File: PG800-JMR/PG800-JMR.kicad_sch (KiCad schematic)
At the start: 51 parts, among them J1 DIN-6, J10 POT_POWER_2, J11 POT_POWER_3, J2 POT_CENTERS_1, J3 POT_CENTERS_2, J4 POT_CENTERS_3, J5 SWITCH_BLK, J6 TEENSY_PIN_BLK1, J7 TEENSY_PIN_BLK3, J8 TEENSY_PIN_BLK2, J9 POT_POWER_1, Q1 BSS138, Q2 BSS138, Q3 BSS138, U1 LM2575-5BT, U2 CD74HC4067M, U3 CD74HC4067M, U4 CD74HC4067M, U5 74HC165A

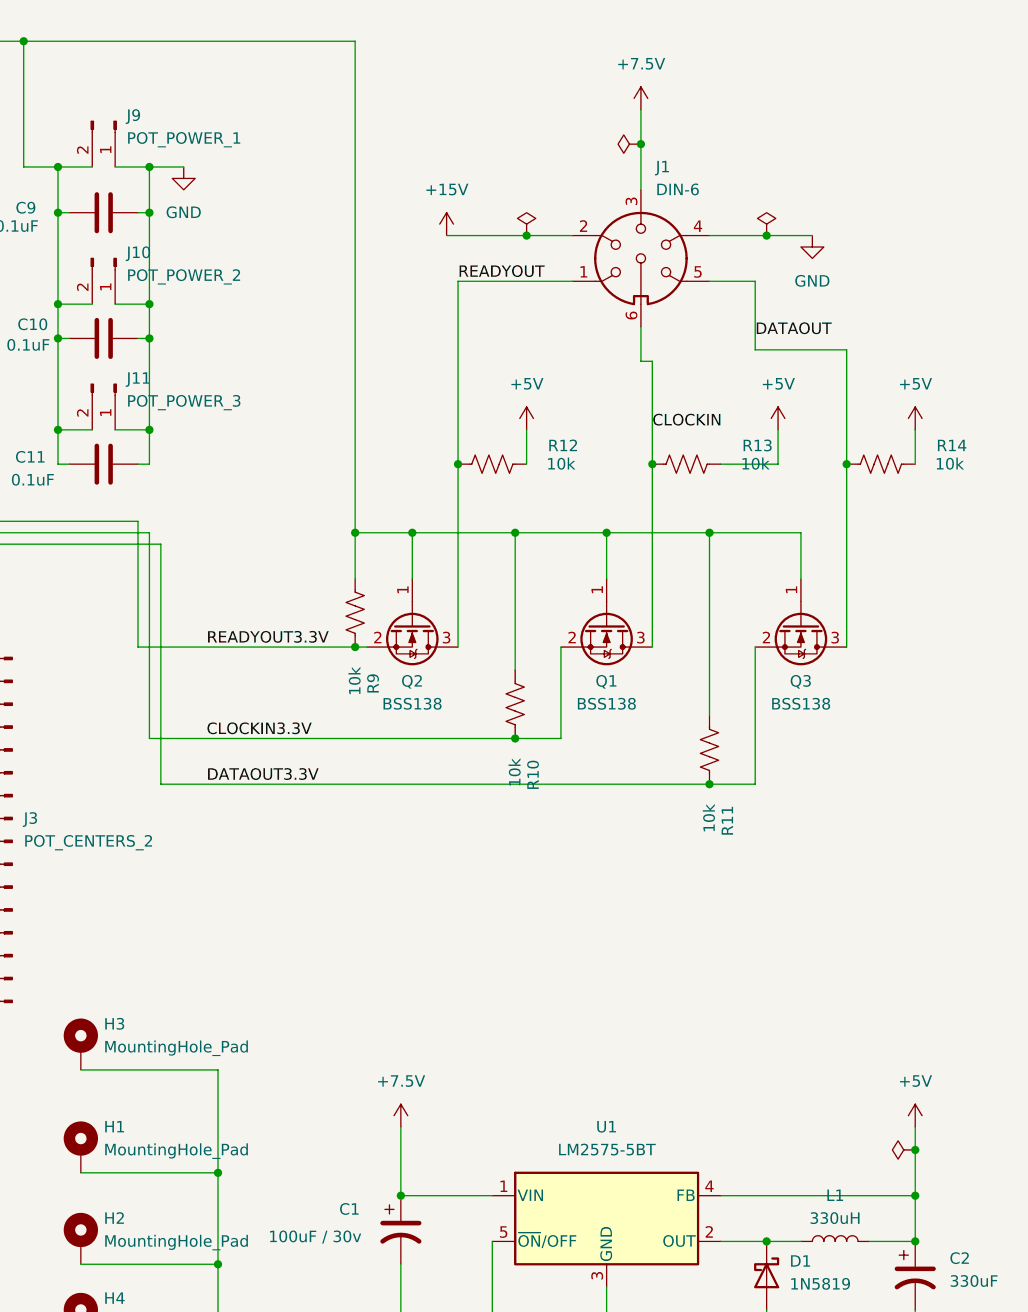
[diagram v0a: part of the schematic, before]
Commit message: updated kicad drawings, tweaked code slightly
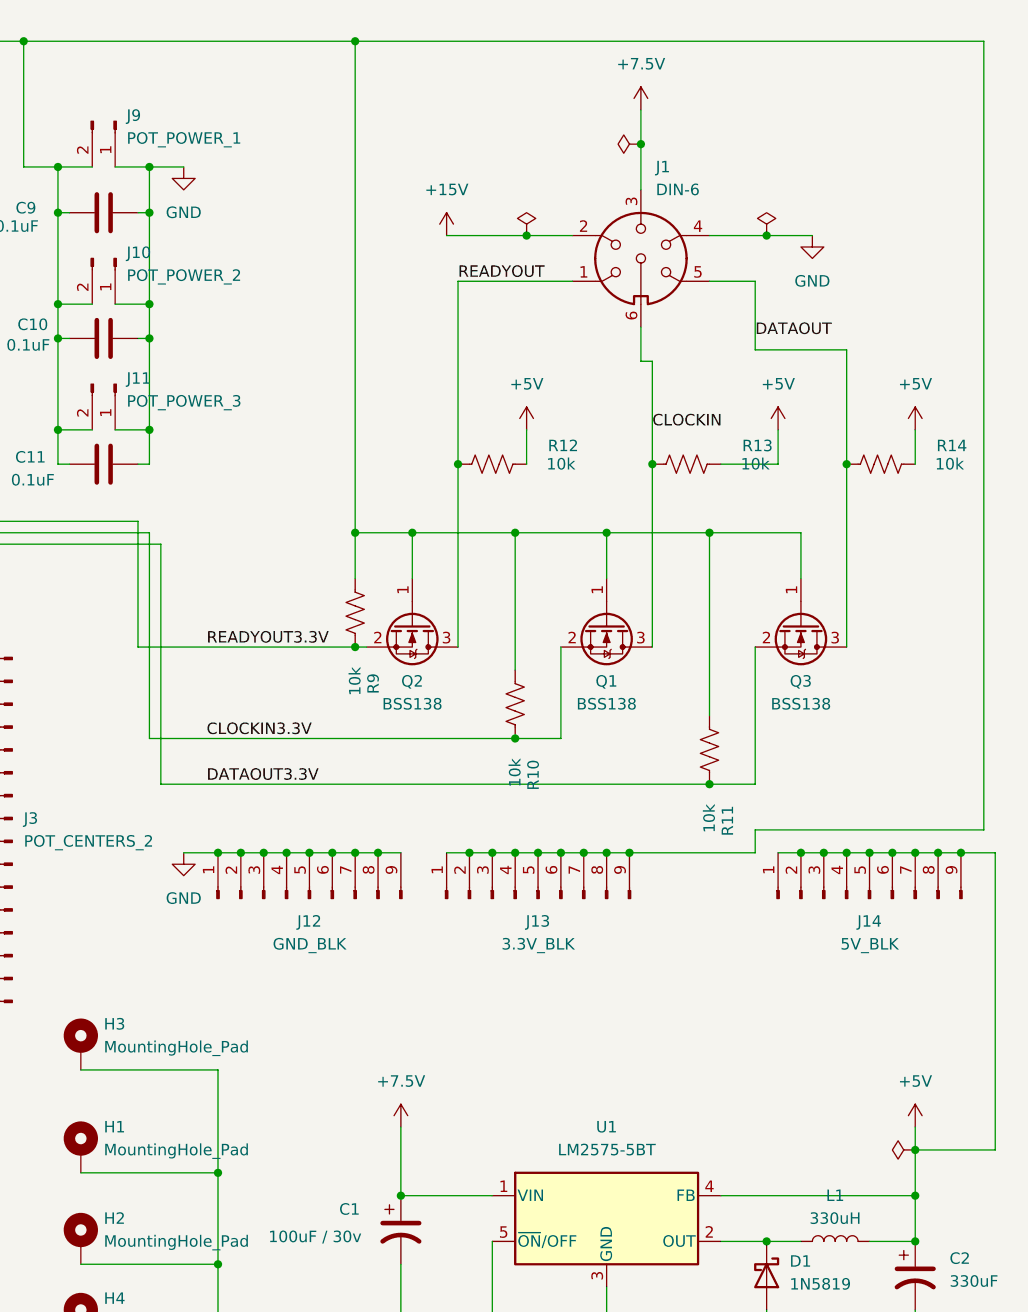
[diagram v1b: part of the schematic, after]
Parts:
- added J12: GND_BLK, Connector_PinHeader_2.54mm:PinHeader_1x09_P2.54mm_Vertical, symbol Connector:Conn_01x09_Pin
- added J13: 3.3V_BLK, Connector_PinHeader_2.54mm:PinHeader_1x09_P2.54mm_Vertical, symbol Connector:Conn_01x09_Pin
- added J14: 5V_BLK, Connector_PinHeader_2.54mm:PinHeader_1x09_P2.54mm_Vertical, symbol Connector:Conn_01x09_Pin
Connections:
- net +5V: now also J14.1 (Pin_1), J14.2 (Pin_2), J14.3 (Pin_3), J14.4 (Pin_4), J14.5 (Pin_5), J14.6 (Pin_6), J14.7 (Pin_7), J14.8 (Pin_8), J14.9 (Pin_9)
- net 3.3V: now also J13.1 (Pin_1), J13.2 (Pin_2), J13.3 (Pin_3), J13.4 (Pin_4), J13.5 (Pin_5), J13.6 (Pin_6), J13.7 (Pin_7), J13.8 (Pin_8), J13.9 (Pin_9)
- net GND: now also J12.1 (Pin_1), J12.2 (Pin_2), J12.3 (Pin_3), J12.4 (Pin_4), J12.5 (Pin_5), J12.6 (Pin_6), J12.7 (Pin_7), J12.8 (Pin_8), J12.9 (Pin_9)
